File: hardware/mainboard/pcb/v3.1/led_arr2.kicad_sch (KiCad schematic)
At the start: 87 parts, among them U3 TPIC6C595, U4 TPIC6C595, U5 TPIC6C595, U6 TPIC6C595, U7 TPIC6C595, U8 TPIC6C595

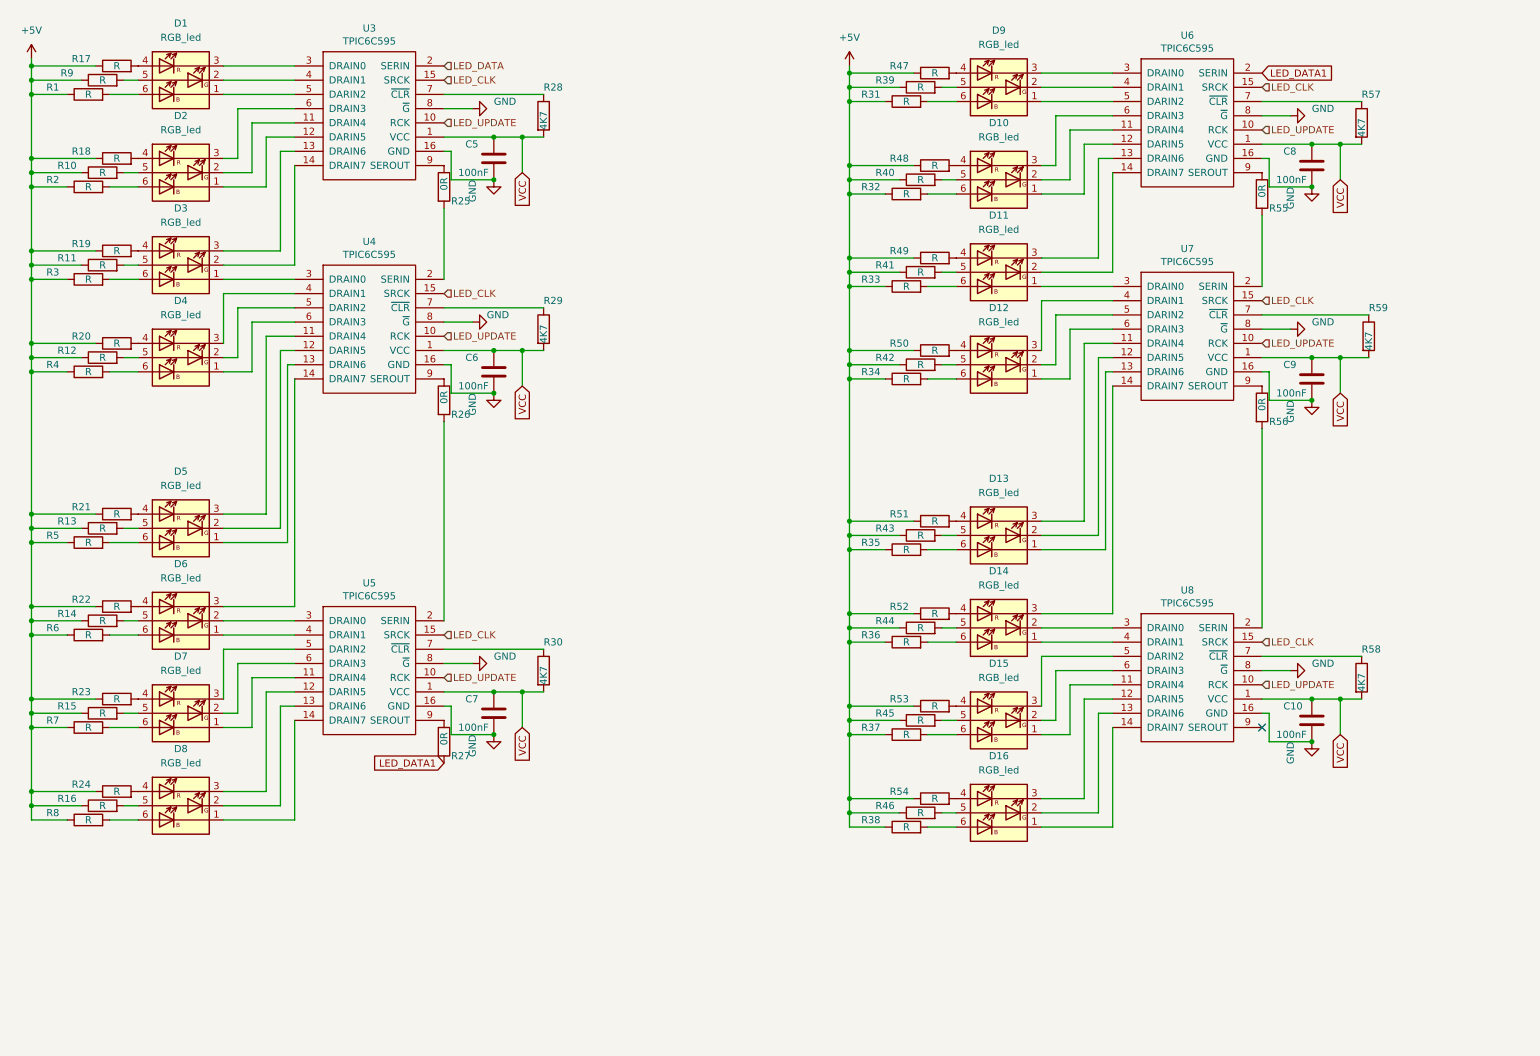
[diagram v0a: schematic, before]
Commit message: .
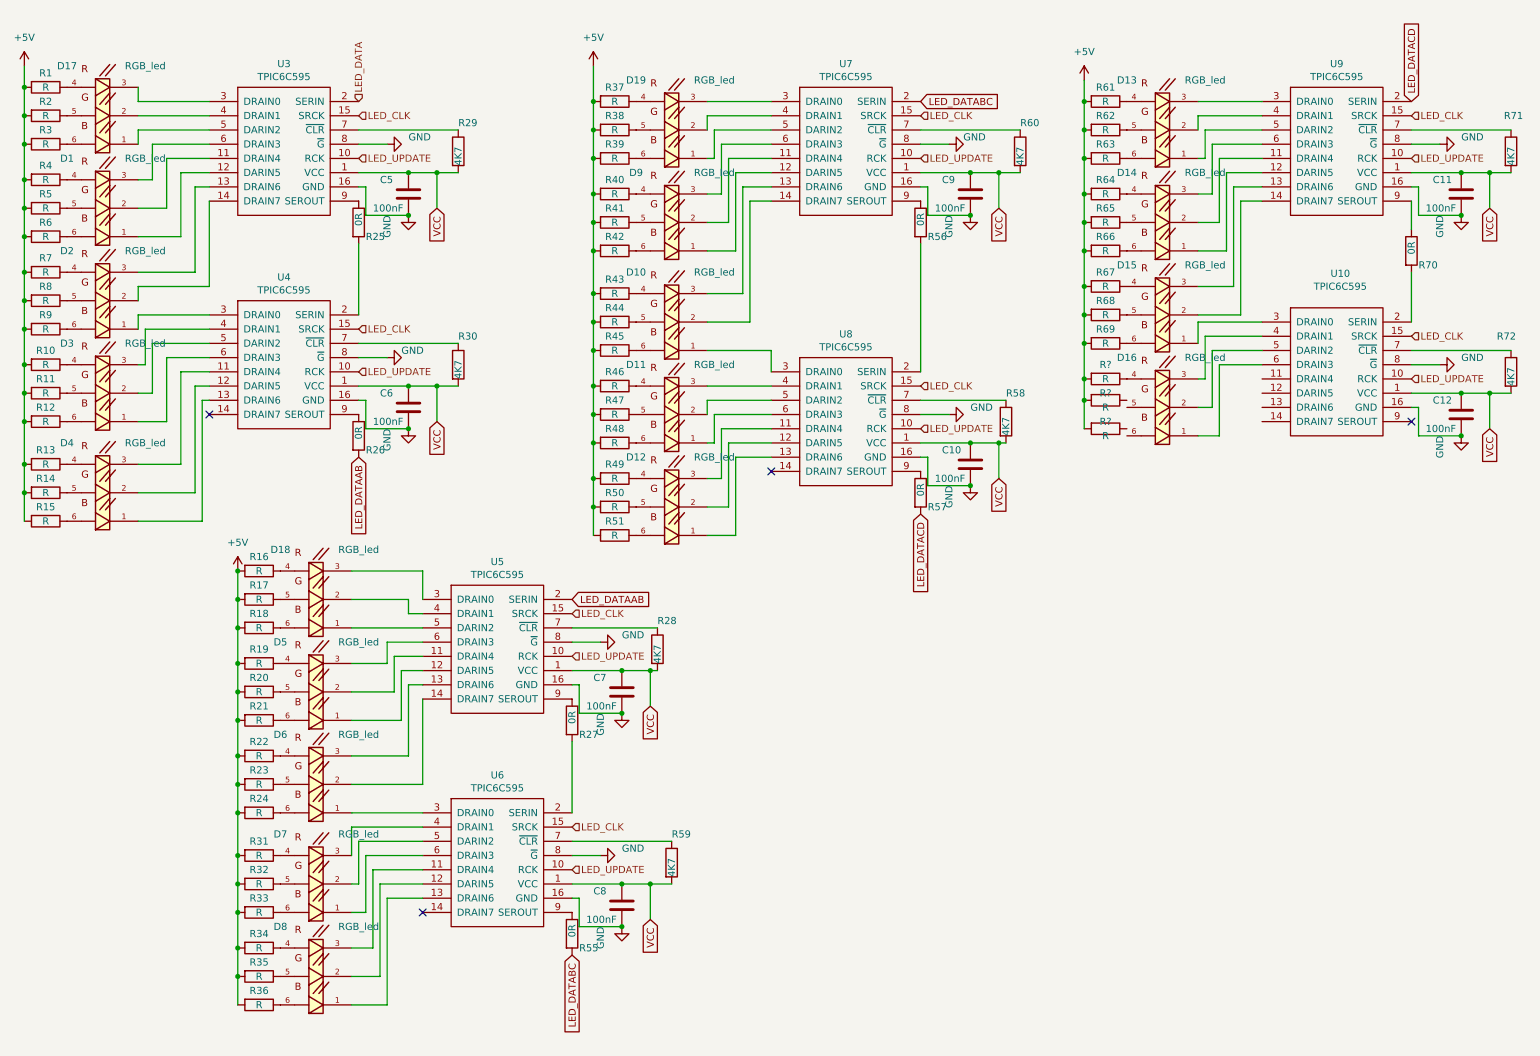
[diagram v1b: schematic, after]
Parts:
- removed D10, D11, D12, D13, D14, D15, D16, D2, D3, D4, D5, D6, D7, D8, D9: RGB_led, LED_SMD:LED_Avago_PLCC6_3x2.8mm, symbol 3dAudioSym:RGB_led
- removed R52, R53, R54: R, Resistor_SMD:R_1206_3216Metric_Pad1.30x1.75mm_HandSolder, symbol Device:R
- added C11, C12: 100nF, Capacitor_SMD:C_1206_3216Metric_Pad1.33x1.80mm_HandSolder, symbol Device:C
- added D10, D11, D12, D13, D14, D15, D16, D17, D18, D19, D2, D3, D4, D5, D6, D7, D8, D9: RGB_led, 3dAudioFoot:LED_QBLP679E-RGB, symbol 3dAudioSym:QBLP679E-RGB
- added R60, R71, R72: 4K7, Resistor_SMD:R_1206_3216Metric_Pad1.30x1.75mm_HandSolder, symbol Device:R
- added R61, R62, R63, R64, R65, R66, R67, R68, R69, R? (x3): R, Resistor_SMD:R_1206_3216Metric, symbol Device:R
- added R70: 0R, Resistor_SMD:R_1206_3216Metric_Pad1.30x1.75mm_HandSolder, symbol Device:R
- added U10, U9: TPIC6C595, Package_SO:SOIC-16_3.9x9.9mm_P1.27mm, symbol 3dAudioSym:TPIC6C595
- D1: footprint LED_SMD:LED_Avago_PLCC6_3x2.8mm -> 3dAudioFoot:LED_QBLP679E-RGB; symbol 3dAudioSym:RGB_led -> 3dAudioSym:QBLP679E-RGB; Check_prices (none) -> https://www.snapeda.com/parts/QBLP679E-RGB/QT+Brightek+%252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; DigiKey_Part_Number (none) -> 1516-1131-2-ND; MANUFACTURER (none) -> QT Brightek; MF (none) -> QT Brightek; MP (none) -> QBLP679E-RGB; Package (none) -> PLCC-6 QT Brightek; Purchase-URL (none) -> https://www.snapeda.com/api/url_track_click_mouser/?unipart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; STANDARD (none) -> Manufacturer Recommendations; SnapEDA_Link (none) -> https://www.snapeda.com/parts/QBLP679E-RGB/QT+Brightek+%252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
- R1, R10, R11, R12, R13, R14, R15, R16, R17, R18, R19, R2, R20, R21, R22, R23, R24, R3, R31, R32, R33, R34, R35, R36, R37, R38, R39, R4, R40, R41, R42, R43, R44, R45, R46, R47, R48, R49, R5, R50, R51, R6, R7, R8, R9: footprint Resistor_SMD:R_1206_3216Metric_Pad1.30x1.75mm_HandSolder -> Resistor_SMD:R_1206_3216Metric
- R57: value 4K7 -> 0R
- renumbered R30 to R28, R28 to R29, R29 to R30
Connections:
- net +5V: now also R1.2, R10.2, R11.2, R12.2, R13.2, R14.2, R15.2, R16.2, R17.2, R18.2, R19.2, R2.2, R20.2, R21.2, R22.2, R23.2, R24.2, R3.2, R31.2, R32.2, R33.2, R34.2, R35.2, R36.2, R37.2, R38.2, R39.2, R4.2, R40.2, R41.2, R42.2, R43.2, R44.2, R45.2, R46.2, R47.2, R48.2, R49.2, R5.2, R50.2, R51.2, R6.2, R7.2, R8.2, R9.2, R61.2, R62.2, R63.2, R64.2, R65.2, R66.2, R67.2, R68.2, R69.2, R?.2, R?.2, R?.2; no longer R1.1, R10.1, R11.1, R12.1, R13.1, R14.1, R15.1, R16.1, R17.1, R18.1, R19.1, R2.1, R20.1, R21.1, R22.1, R23.1, R24.1, R3.1, R31.1, R32.1, R33.1, R34.1, R35.1, R36.1, R37.1, R38.1, R39.1, R4.1, R40.1, R41.1, R42.1, R43.1, R44.1, R45.1, R46.1, R47.1, R48.1, R49.1, R5.1, R50.1, R51.1, R6.1, R7.1, R8.1, R9.1
- net GND: now also C11.2, C12.2, U10.16 (GND), U10.8 (~{G}), U9.16 (GND), U9.8 (~{G})
- net LED_CLK: now also U10.15 (SRCK), U9.15 (SRCK)
- net LED_UPDATE: now also U10.10 (RCK), U9.10 (RCK)
- net VCC: now also C11.1, C12.1, R60.2, R71.2, R72.2, U10.1 (VCC), U9.1 (VCC); no longer R57.2
- net at U5.11 (DRAIN4): now also D5.2
- net at U5.12 (DARIN5): now also D5.1
- net at U5.13 (DRAIN6): now also D6.3
- net at U5.14 (DRAIN7): now also D6.2
- net LED_DATAAB: now reaches R26.2, U5.2 (SERIN)
- net at U5.3 (DRAIN0): now also D18.3
- net at U5.4 (DRAIN1): now also D18.2
- net at U5.5 (DARIN2): now also D18.1
- net at U5.6 (DRAIN3): now also D5.3
- net at U4.13 (DRAIN6): now also D4.1
- net at U4.12 (DARIN5): now also D4.2
- net at U4.11 (DRAIN4): now also D4.3
- net at U8.4 (DRAIN1): now also D11.3
- net at U8.3 (DRAIN0): now also D10.1
- net at U7.14 (DRAIN7): now also D10.2
- net at U4.3 (DRAIN0): now also D2.1
- net at U3.14 (DRAIN7): now also D2.2
- net at U3.13 (DRAIN6): now also D2.3
- net LED_DATABC: now reaches R55.2, U7.2 (SERIN)
- net at U6.7 (~{CLR}): now also R59.1; no longer R57.1
- net at U4.6 (DRAIN3): now also D3.1
- net at U4.5 (DARIN2): now also D3.2
- net at U4.4 (DRAIN1): now also D3.3
- net at U8.13 (DRAIN6): now also D12.1
- net at U8.12 (DARIN5): now also D12.2
- net at U7.3 (DRAIN0): now also D19.3
- net at U6.13 (DRAIN6): now also D8.1
- net at U7.7 (~{CLR}): now also R60.1; no longer R59.1
- net at U7.6 (DRAIN3): now also D9.3
- net at U7.5 (DARIN2): now also D19.1
- net at U7.4 (DRAIN1): now also D19.2
- net at U3.12 (DARIN5): now also D1.1
- net at U3.11 (DRAIN4): now also D1.2
- net at U3.6 (DRAIN3): now also D1.3
- net at D1.5: now also R5.1; no longer R9.2
- net at U3.5 (DARIN2): now also D17.1; no longer D1.1 (KB)
- net at U3.4 (DRAIN1): now also D17.2; no longer D1.2 (KG)
- net at U3.3 (DRAIN0): now also D17.3; no longer D1.3 (KR)
- net at D1.4: now also R4.1; no longer R17.2
- net at D1.6: now also R6.1; no longer R1.2
- net at U7.11 (DRAIN4): now also D9.2
- net at U7.12 (DARIN5): now also D9.1
- net at U7.13 (DRAIN6): now also D10.3
- net at U8.11 (DRAIN4): now also D12.3
- net at U8.5 (DARIN2): now also D11.2
- net at U8.6 (DRAIN3): now also D11.1
- net at U8.9 (SEROUT): now also R57.1
- net at U6.12 (DARIN5): now also D8.2
- net at U6.11 (DRAIN4): now also D8.3
- net at U6.6 (DRAIN3): now also D7.1
- net at U6.5 (DARIN2): now also D7.2
- net at U6.4 (DRAIN1): now also D7.3
- net at U6.3 (DRAIN0): now also D6.1
- net LED_DATA1: no longer names the net of R27.2, U6.2 (SERIN)
- new net: D16.4, R?.1
- new net: R70.1, U9.9 (SEROUT)
- new net: R70.2, U10.2 (SERIN)
- new net: D7.6, R33.1
- new net: D18.5, R17.1
- new net: D14.2, U9.11 (DRAIN4)
- new net: D14.1, U9.12 (DARIN5)
- new net: D15.3, U9.13 (DRAIN6)
- new net: D15.2, U9.14 (DRAIN7)
- new net: D13.3, U9.3 (DRAIN0)
- new net: D13.2, U9.4 (DRAIN1)
- new net: D13.1, U9.5 (DARIN2)
- new net: D14.3, U9.6 (DRAIN3)
- new net: R71.1, U9.7 (~{CLR})
- new net: D7.5, R32.1
- new net: D3.4, R10.1
- new net: D3.5, R11.1
- new net: D3.6, R12.1
- new net: D11.6, R48.1
- new net: D5.4, R19.1
- new net: D5.5, R20.1
- new net: D5.6, R21.1
- new net: D15.6, R69.1
- new net: D4.5, R14.1
- new net: D6.4, R22.1
- new net: D12.4, R49.1
- new net: D10.4, R43.1
- new net: D11.4, R46.1
- new net: D11.5, R47.1
- new net: D4.4, R13.1
- new net: D4.6, R15.1
- new net: D8.6, R36.1
- new net: D13.4, R61.1
- new net: D13.5, R62.1
- new net: D13.6, R63.1
- new net: D7.4, R31.1
- new net: D18.4, R16.1
- new net: D18.6, R18.1
- new net: D9.4, R40.1
- new net: D9.5, R41.1
- new net: D9.6, R42.1
- new net: D14.5, R65.1
- new net: R72.1, U10.7 (~{CLR})
- new net: D14.6, R66.1
- new net: D19.4, R37.1
- new net: D19.5, R38.1
- new net: D19.6, R39.1
- new net: D2.6, R9.1
- new net: D15.1, U10.3 (DRAIN0)
- new net: D16.3, U10.4 (DRAIN1)
- new net: D16.2, U10.5 (DARIN2)
- new net: D16.1, U10.6 (DRAIN3)
- new net: D14.4, R64.1
- new net: D12.5, R50.1
- new net: D12.6, R51.1
- new net: D17.4, R1.1
- new net: D17.5, R2.1
- new net: D17.6, R3.1
- new net: D6.5, R23.1
- new net: D6.6, R24.1
- new net: D2.5, R8.1
- new net: D8.4, R34.1
- new net: D2.4, R7.1
- new net: D8.5, R35.1
- new net: D15.4, R67.1
- new net: D10.5, R44.1
- new net: D10.6, R45.1
- new net: D15.5, R68.1
- new net LED_DATACD: R57.2, U9.2 (SERIN)
- no-connect marks 1 -> 4
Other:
- moved on the sheet: C5, C6, C7, R25, R26, R27, R28, R29, R30, U3, U4, U5
